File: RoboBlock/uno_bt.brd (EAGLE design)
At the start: 100 x 80 mm, 17 parts, among them IC1 L293D, U1 ARDUINOR3-DIMENSION

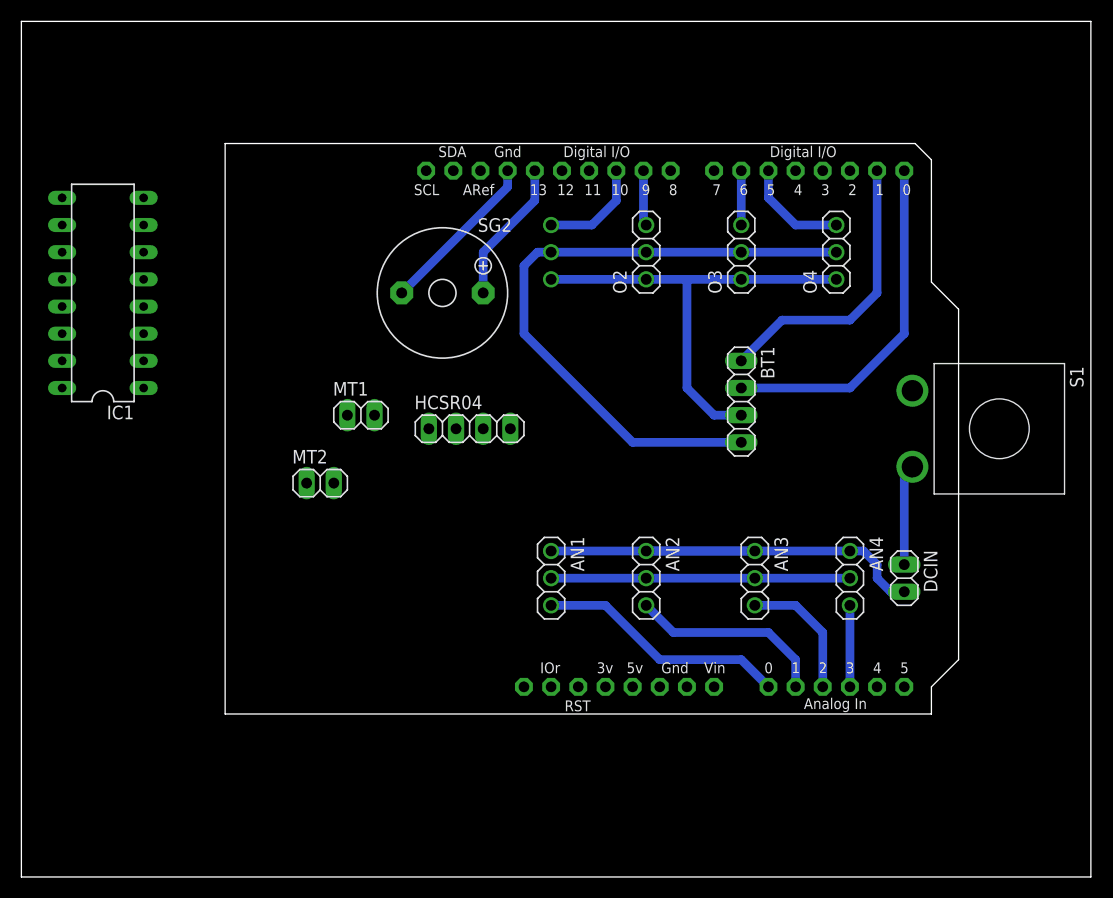
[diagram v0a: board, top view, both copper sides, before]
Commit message: sensor
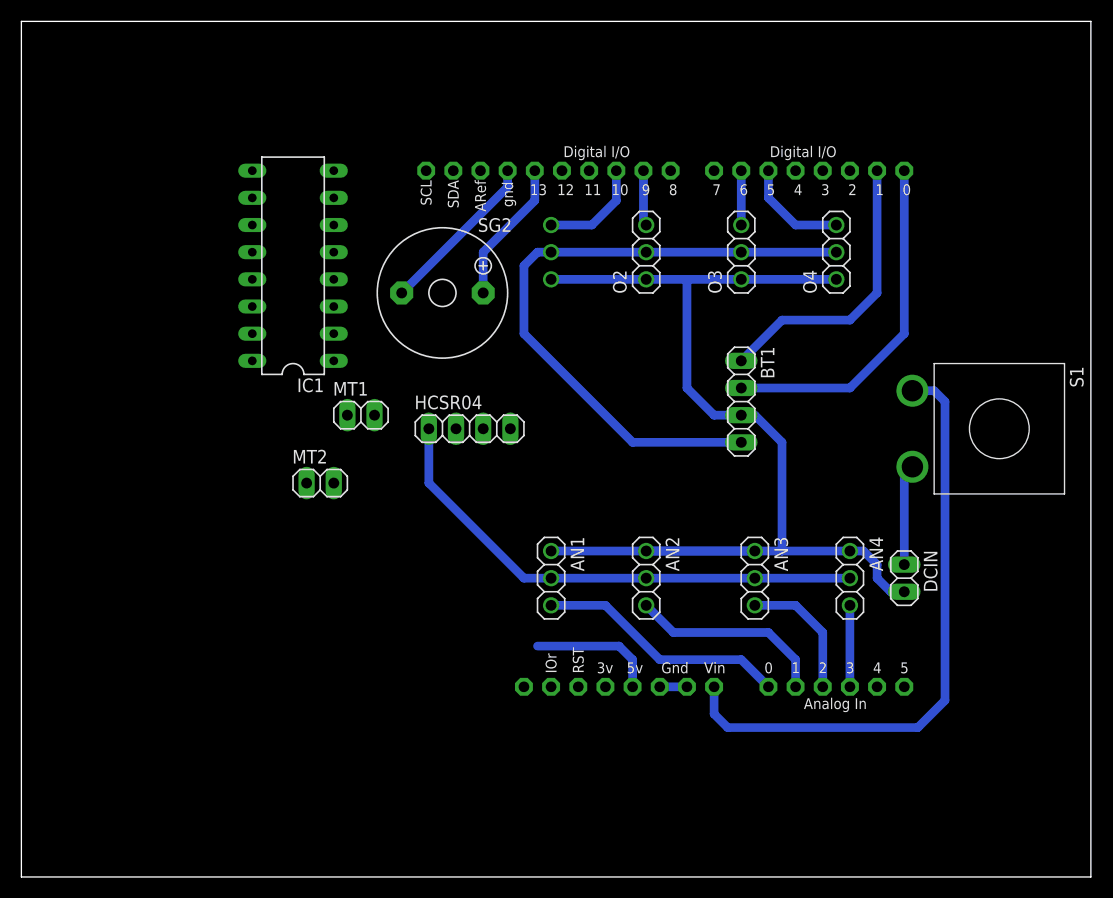
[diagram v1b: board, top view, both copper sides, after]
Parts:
- U1: value ARDUINOR3-DIMENSION -> ARDUINOR3-BPLACE; device adafruit_arduino:ARDUINOR3 -> adafruit_arduino:ARDUINOR3-BPLACE
- moved IC1 18.0 mm to (25.4, 57.1)
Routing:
- net VIN: track 0.00 -> 69.1 mm
- net VCC: track 88.6 -> 108.7 mm
- net GND: track 104.0 -> 121.6 mm
